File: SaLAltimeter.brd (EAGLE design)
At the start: 74.6 x 19.7 mm, 91 parts, among them U1 ATSAMD21G-A, U2 V_REG_LDOSMD, U3 ADXL345, Y3 32MHz

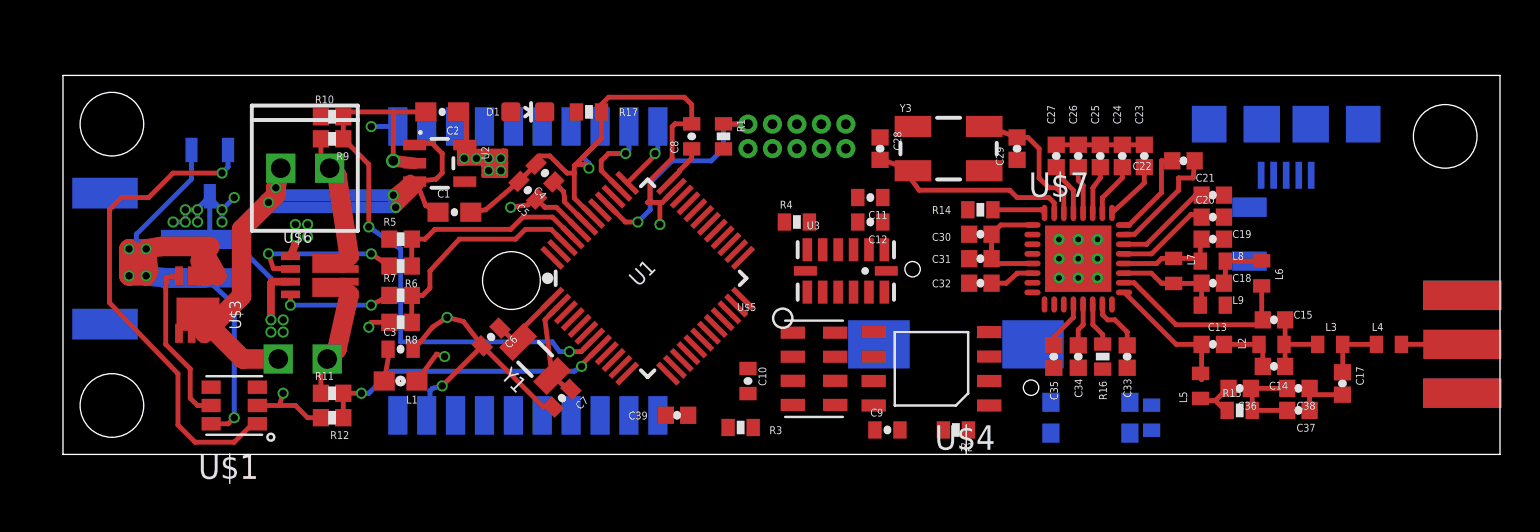
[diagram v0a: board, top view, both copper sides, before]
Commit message: finshed wiring
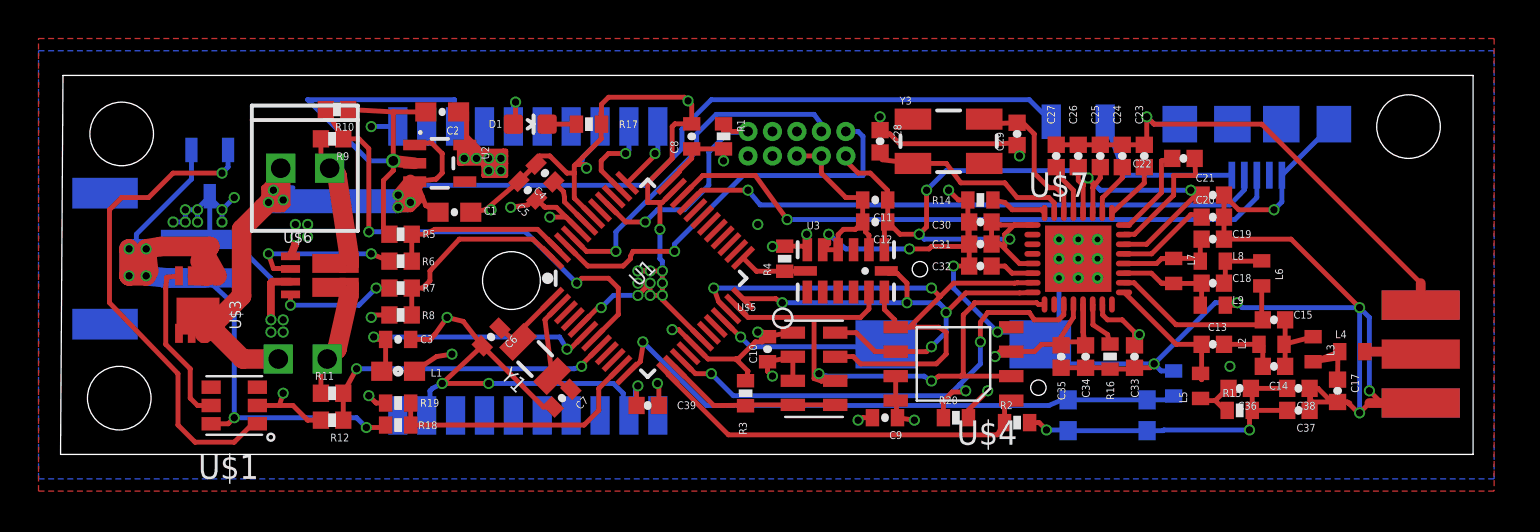
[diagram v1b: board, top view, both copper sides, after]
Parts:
- added R18: 100k, SparkFun-Passives:0402-RES
- added R19: 27k, SparkFun-Passives:0402-RES
- added R20: 10k, SparkFun-Passives:0402-RES
- C8: value (none) -> 0.1uF
- J1: value (none) -> BAT
- JP2: value (none) -> MAIN
- JP3: value (none) -> DROGUE
- R1, R13, R2, R3, R4: value (none) -> 10k
- R15: value (none) -> 18
- U4: value (none) -> gps
- Y1: value (none) -> 32.768kHx
- moved F1 10.6 mm to (48.3, 17.3), turned to 0 degrees
- moved R2 3.20 mm to (45.1, 1.65), turned to 0 degrees
- moved J$1 2.22 mm to (66.0, 2.67)
- moved R13 2.11 mm to (53.2, 3.68), turned to 270 degrees
- moved R4 2.01 mm to (33.0, 10.2), turned to 90 degrees
- moved STANDOFF1 1.97 mm to (65.4, 17.0)
- moved L4 1.94 mm to (62.5, 5.33)
- moved C10 1.94 mm to (32.1, 5.46), turned to 270 degrees
- moved R3 1.80 mm to (31.0, 3.17), turned to 90 degrees
- moved C39 1.61 mm to (25.9, 2.54), turned to 0 degrees
- moved JP4 1.52 mm to (57.5, 17.1)
- moved U$4 1.17 mm to (41.8, 5.33)
- moved L3 0.92 mm to (60.5, 5.46), turned to 270 degrees
- moved S2 0.90 mm to (49.8, 2.03)
- moved C32 0.89 mm to (43.2, 9.78)
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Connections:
- removed net N$7: U1.6
- net BUZZER: now also SG1.+, U1.21; no longer SG1.-, U1.27
- net CS_ACCEL: now also U1.25; no longer U1.24
- net CS_BARO: now also U1.14; no longer U1.22
- net CS_MEM: now also U1.13; no longer U1.23
- net CS_TX: now also R20.1, U1.15; no longer U1.28
- net FIRE_A: now also U1.47; no longer U1.45
- net FIRE_B: now also U1.48; no longer U1.46
- net GND: now also R19.1, R20.2, SG1.-, U$7.EXP, U$7.EXP@1, U$7.EXP@2, U$7.EXP@3, U$7.EXP@4, U$7.EXP@5, U$7.EXP@6, U$7.EXP@7, U$7.EXP@8, U$7.EXP@9; no longer SG1.+
- net LVD_IN: now also F1.2
- net N$5: now also U1.6
- net PROG: now also U1.12; no longer U1.29
- net RAW: now also R18.2
- net SENSE_BAT: now also R18.1, R19.2, U1.11; no longer U1.9
- net SPI_MISO: now also U1.23; no longer U1.21, U1.25
- net SPI_MOSI: now also U1.22; no longer U1.19, U1.26
- net SPI_SCK: now also U1.24; no longer U1.20
- net SWCLK: now also U1.45
- net SWDIO: now also U1.46
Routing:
- net GND: track 121.0 -> 383.4 mm, vias 23 -> 57
- net 3.3V: track 81.4 -> 232.9 mm, vias 9 -> 26
- net LVD_IN: track 36.8 -> 101.6 mm, vias 4 -> 6
- net USB_D+: track 0.00 -> 33.1 mm, vias 0 -> 1
- net SPI_MOSI: track 0.00 -> 32.8 mm, vias 0 -> 2
- net PROG: track 0.00 -> 31.3 mm, vias 0 -> 1
- net SPI_MISO: track 0.00 -> 30.8 mm, vias 0 -> 2
- net USB_D-: track 0.00 -> 30.6 mm, vias 0 -> 1
- net CS_TX: track 0.00 -> 27.2 mm, vias 0 -> 3
- net SPI_SCK: track 0.00 -> 25.8 mm, vias 0 -> 4
- net SWDIO: track 0.00 -> 21.2 mm, vias 0 -> 1
- net CS_MEM: track 0.00 -> 20.5 mm
- net SWCLK: track 0.00 -> 17.9 mm, vias 0 -> 1
- net SENSE_BAT: track 0.00 -> 14.0 mm
- net N$5: track 1.68 -> 14.2 mm, vias 0 -> 2
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- added copper zone on layer 15, net 3.3V
- added copper zone on layer 1, net GND
- added copper zone on layer 16, net GND
- added copper zone on layer 2, net GND
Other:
- board size 74.6 x 19.7 mm -> 73.3 x 19.7 mm
